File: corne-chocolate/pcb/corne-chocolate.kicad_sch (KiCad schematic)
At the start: 81 parts, among them J1 MJ-4PP-9, J2 Conn_01x04, J3 Conn_01x03, P1 Conn_01x01, P2 Conn_01x01, SW10 SW_PUSH, SW11 SW_PUSH, SW12 SW_PUSH, SW14 SW_PUSH, SW15 SW_PUSH, SW16 SW_PUSH, SW17 SW_PUSH, SW18 SW_PUSH, SW19 SW_PUSH, SW2 SW_PUSH, SW20 SW_PUSH, SW21 SW_PUSH, SW3 SW_PUSH, SW4 SW_PUSH, SW5 SW_PUSH, SW6 SW_PUSH, SW8 SW_PUSH, SW9 SW_PUSH, U1 ProMicro

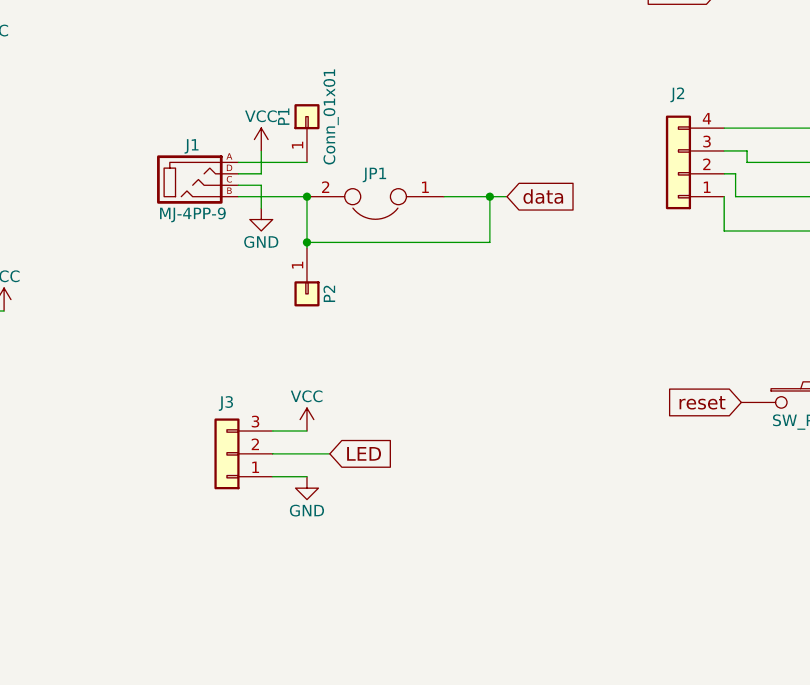
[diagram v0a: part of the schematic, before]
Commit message: reannotates
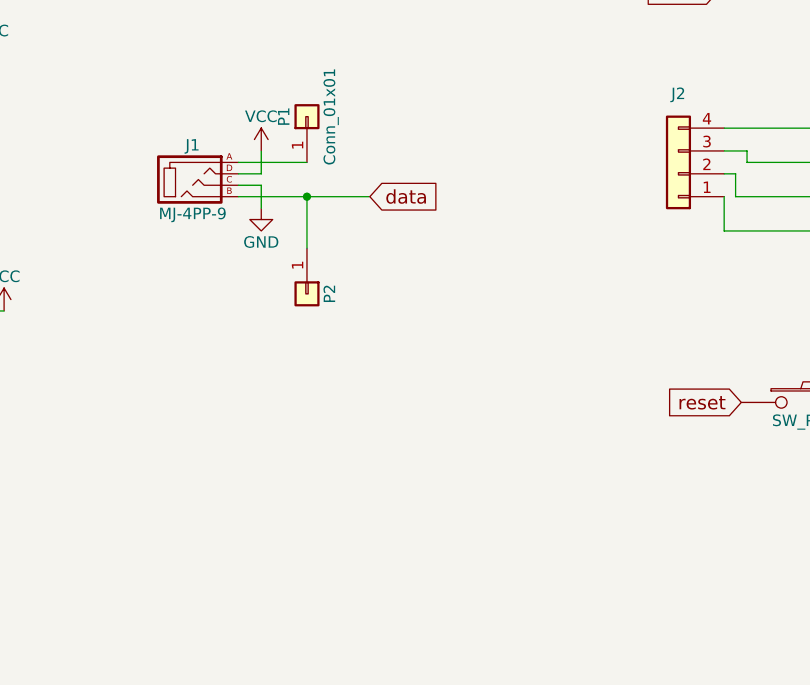
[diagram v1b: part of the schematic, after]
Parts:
- removed J3: Conn_01x03, kbd:StripLED_1side, symbol Connector_Generic:Conn_01x03
- removed JP1: Device:Jumper, kbd:Jumper, symbol kbd:Jumper-Device
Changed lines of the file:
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@@
   (junction (at 94.615 145.415) (diameter 0) (color 0 0 0 0)
   )
+  (junction (at 167.64 108.585) (diameter 0) (color 0 0 0 0)
+  )
   (junction (at 79.375 145.415) (diameter 0) (color 0 0 0 0)
   )
@@
   (junction (at 94.615 163.195) (diameter 0) (color 0 0 0 0)
   )
-  (junction (at 187.96 108.585) (diameter 0) (color 0 0 0 0)
-  )
   (junction (at 109.855 170.815) (diameter 0) (color 0 0 0 0)
   )
@@
   (junction (at 201.93 47.625) (diameter 0) (color 0 0 0 0)
   )
-  (junction (at 167.64 108.585) (diameter 0) (color 0 0 0 0)
-  )
   (junction (at 94.615 132.715) (diameter 0) (color 0 0 0 0)
   )
   (junction (at 92.075 107.315) (diameter 0) (color 0 0 0 0)
   )
-  (junction (at 167.64 113.665) (diameter 0) (color 0 0 0 0)
-  )
   (junction (at 217.17 55.245) (diameter 0) (color 0 0 0 0)
   )
@@
     (stroke (width 0) (type default))
   )
-  (wire (pts (xy 167.64 113.665) (xy 167.64 114.3))
+  (wire (pts (xy 167.64 108.585) (xy 167.64 114.3))
     (stroke (width 0) (type default))
   )
@@
     (stroke (width 0) (type default))
   )
-  (wire (pts (xy 167.64 108.585) (xy 167.64 113.665))
-    (stroke (width 0) (type default))
-  )
   (wire (pts (xy 92.075 154.305) (xy 92.075 150.495))
     (stroke (width 0) (type default))
@@
     (stroke (width 0) (type default))
   )
-  (wire (pts (xy 187.96 108.585) (xy 182.88 108.585))
+  (wire (pts (xy 167.64 108.585) (xy 174.625 108.585))
     (stroke (width 0) (type default))
   )
@@
     (stroke (width 0) (type default))
   )
-  (wire (pts (xy 163.83 134.62) (xy 167.64 134.62))
-    (stroke (width 0) (type default))
-  )
   (wire (pts (xy 112.395 170.815) (xy 112.395 167.005))
     (stroke (width 0) (type default))
@@
     (stroke (width 0) (type default))
   )
-  (wire (pts (xy 187.96 113.665) (xy 167.64 113.665))
-    (stroke (width 0) (type default))
-  )
   (wire (pts (xy 76.835 158.115) (xy 79.375 158.115))
     (stroke (width 0) (type default))
@@
     (stroke (width 0) (type default))
   )
-  (wire (pts (xy 163.83 137.16) (xy 170.18 137.16))
-    (stroke (width 0) (type default))
-  )
   (wire (pts (xy 79.375 150.495) (xy 79.375 158.115))
     (stroke (width 0) (type default))
@@
     (stroke (width 0) (type default))
   )
-  (wire (pts (xy 187.96 108.585) (xy 187.96 113.665))
-    (stroke (width 0) (type default))
-  )
   (wire (pts (xy 48.26 97.155) (xy 48.26 111.76))
     (stroke (width 0) (type default))
@@
     (stroke (width 0) (type default))
   )
-  (wire (pts (xy 163.83 139.7) (xy 167.64 139.7))
-    (stroke (width 0) (type default))
-  )
-  (wire (pts (xy 189.865 108.585) (xy 187.96 108.585))
-    (stroke (width 0) (type default))
-  )
   (wire (pts (xy 102.87 97.155) (xy 102.87 102.235))
     (stroke (width 0) (type default))
@@
     )
   )
-  (global_label "data" (shape input) (at 189.865 108.585 0) (fields_autoplaced)
+  (global_label "data" (shape input) (at 174.625 108.585 0) (fields_autoplaced)
     (effects (font (size 1.524 1.524)) (justify left))
-    (property "Intersheetrefs" "${INTERSHEET_REFS}" (at 197.6694 108.585 0)
+    (property "Intersheetrefs" "${INTERSHEET_REFS}" (at 182.4294 108.585 0)
       (effects (font (size 1.27 1.27)) (justify left) hide)
     )
@@
     )
   )
-  (global_label "LED" (shape input) (at 170.18 137.16 0) (fields_autoplaced)
-    (effects (font (size 1.524 1.524)) (justify left))
-    (property "Intersheetrefs" "${INTERSHEET_REFS}" (at 177.1134 137.16 0)
-      (effects (font (size 1.27 1.27)) (justify left) hide)
-    )
-  )
   (global_label "SDA" (shape input) (at 50.165 57.15 180) (fields_autoplaced)
     (effects (font (size 1.1938 1.1938)) (justify right))
@@
     )
   )
-  (symbol (lib_id "Connector_Generic:Conn_01x03") (at 158.75 137.16 180) (unit 1)
-    (in_bom yes) (on_board yes) (dnp no)
-    (property "Reference" "J3" (at 158.75 131.445 0)
-      (effects (font (size 1.27 1.27)))
-    )
-    (property "Value" "Conn_01x03" (at 158.75 132.08 0)
-      (effects (font (size 1.27 1.27)) hide)
-    )
-    (property "Footprint" "kbd:StripLED_1side" (at 158.75 137.16 0)
-      (effects (font (size 1.27 1.27)) hide)
-    )
-    (property "Datasheet" "~" (at 158.75 137.16 0)
-      (effects (font (size 1.27 1.27)) hide)
-    )
-    (property "supplier" "" (at 158.75 137.16 0)
-      (effects (font (size 1.27 1.27)) hide)
-    )
-    (property "supplier pn" "" (at 158.75 137.16 0)
-      (effects (font (size 1.27 1.27)) hide)
-    )
-    (pin "1")
-    (pin "2")
-    (pin "3")
-    (instances
-      (project "corne-chocolate"
-        (path "/b2404ab0-025a-473e-9fbb-0abc932972cf"
-          (reference "J3") (unit 1)
-        )
-      )
-    )
-  )
-  (symbol (lib_id "power:VCC") (at 167.64 134.62 0) (unit 1)
-    (in_bom yes) (on_board yes) (dnp no)
-    (property "Reference" "#PWR024" (at 167.64 138.43 0)
-      (effects (font (size 1.27 1.27)) hide)
-    )
-    (property "Value" "VCC" (at 167.64 130.81 0)
-      (effects (font (size 1.27 1.27)))
-    )
-    (property "Footprint" "" (at 167.64 134.62 0)
-      (effects (font (size 1.27 1.27)) hide)
-    )
-    (property "Datasheet" "" (at 167.64 134.62 0)
-      (effects (font (size 1.27 1.27)) hide)
-    )
-    (pin "1")
-    (instances
-      (project "corne-chocolate"
-        (path "/b2404ab0-025a-473e-9fbb-0abc932972cf"
-          (reference "#PWR024") (unit 1)
-        )
-      )
-    )
-  )
-  (symbol (lib_id "power:GND") (at 167.64 139.7 0) (unit 1)
-    (in_bom yes) (on_board yes) (dnp no)
-    (property "Reference" "#PWR025" (at 167.64 146.05 0)
-      (effects (font (size 1.27 1.27)) hide)
-    )
-    (property "Value" "GND" (at 167.64 143.51 0)
-      (effects (font (size 1.27 1.27)))
-    )
-    (property "Footprint" "" (at 167.64 139.7 0)
-      (effects (font (size 1.27 1.27)) hide)
-    )
-    (property "Datasheet" "" (at 167.64 139.7 0)
-      (effects (font (size 1.27 1.27)) hide)
-    )
-    (pin "1")
-    (instances
-      (project "corne-chocolate"
-        (path "/b2404ab0-025a-473e-9fbb-0abc932972cf"
-          (reference "#PWR025") (unit 1)
-        )
-      )
-    )
-  )
   (symbol (lib_id "kbd:MJ-4PP-9") (at 154.94 106.68 0) (unit 1)
     (in_bom yes) (on_board yes) (dnp no)
@@
         )
       )
-    )
-  )
-  (symbol (lib_id "kbd:Jumper-Device") (at 175.26 108.585 180) (unit 1)
-    (in_bom yes) (on_board yes) (dnp no) (fields_autoplaced)
-    (property "Reference" "JP1" (at 175.26 106.045 0)
-      (effects (font (size 1.27 1.27)))
-    )
-    (property "Value" "Device:Jumper" (at 175.26 106.553 0)
-      (effects (font (size 1.27 1.27)) hide)
-    )
-    (property "Footprint" "kbd:Jumper" (at 175.26 108.585 0)
-      (effects (font (size 1.27 1.27)) hide)
-    )
-    (property "Datasheet" "" (at 175.26 108.585 0)
-      (effects (font (size 1.27 1.27)) hide)
-    )
-    (property "supplier" "" (at 175.26 108.585 0)
-      (effects (font (size 1.27 1.27)) hide)
-    )
-    (property "supplier pn" "" (at 175.26 108.585 0)
-      (effects (font (size 1.27 1.27)) hide)
-    )
-    (pin "1")
-    (pin "2")
-    (instances
-      (project "corne-chocolate"
-        (path "/b2404ab0-025a-473e-9fbb-0abc932972cf"
-          (reference "JP1") (unit 1)
-        )
-      )
